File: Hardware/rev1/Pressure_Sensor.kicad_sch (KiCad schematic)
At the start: 4 parts, among them U3 MS5607-02BA

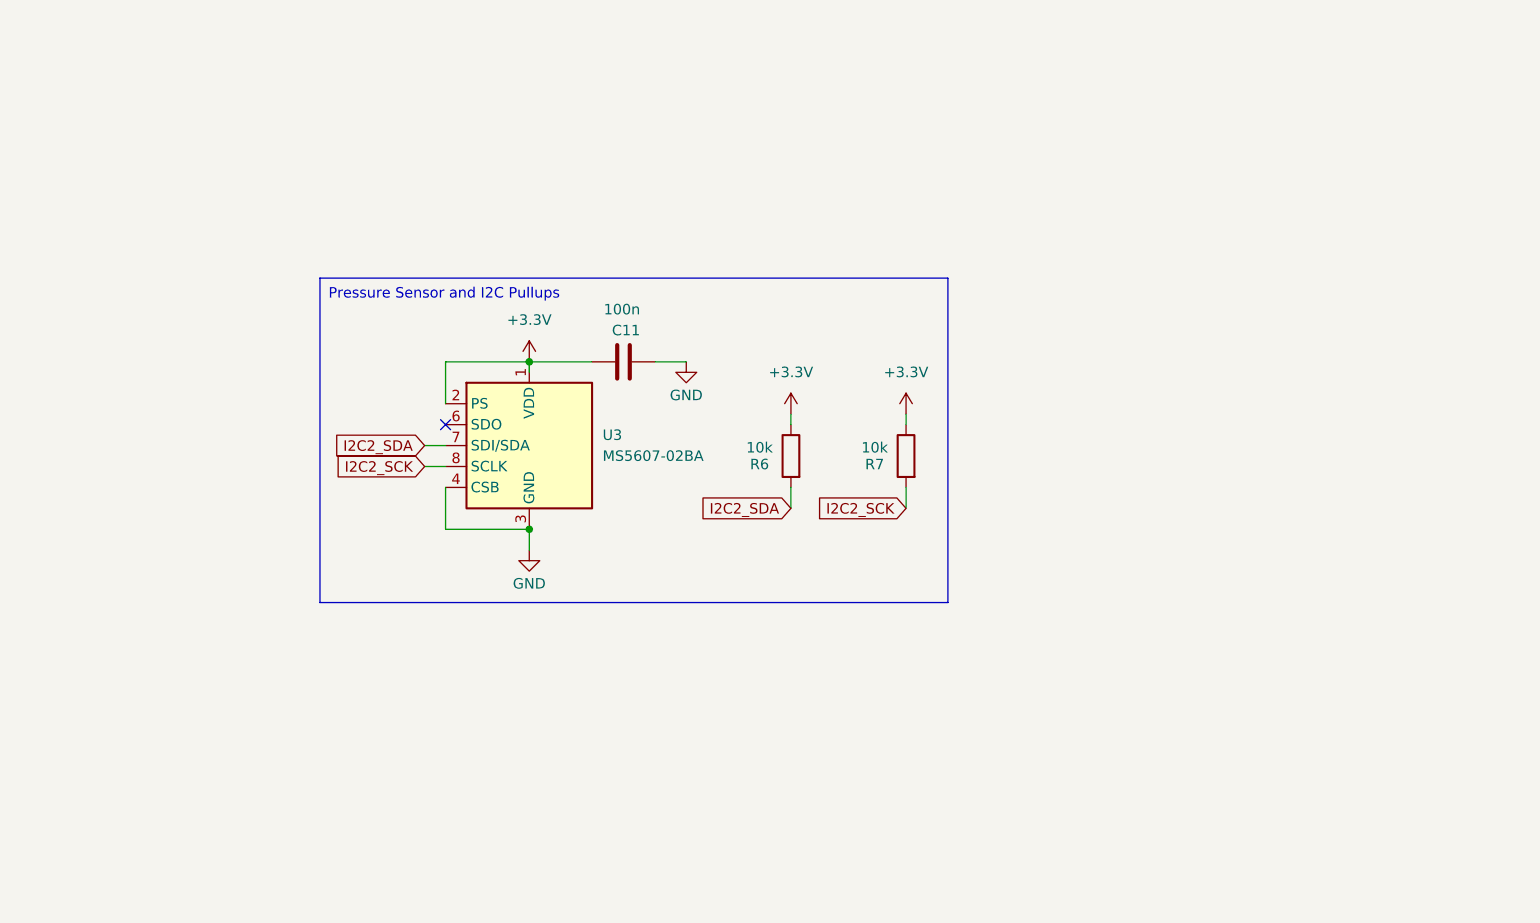
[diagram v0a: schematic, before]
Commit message: Add buses (maybe)
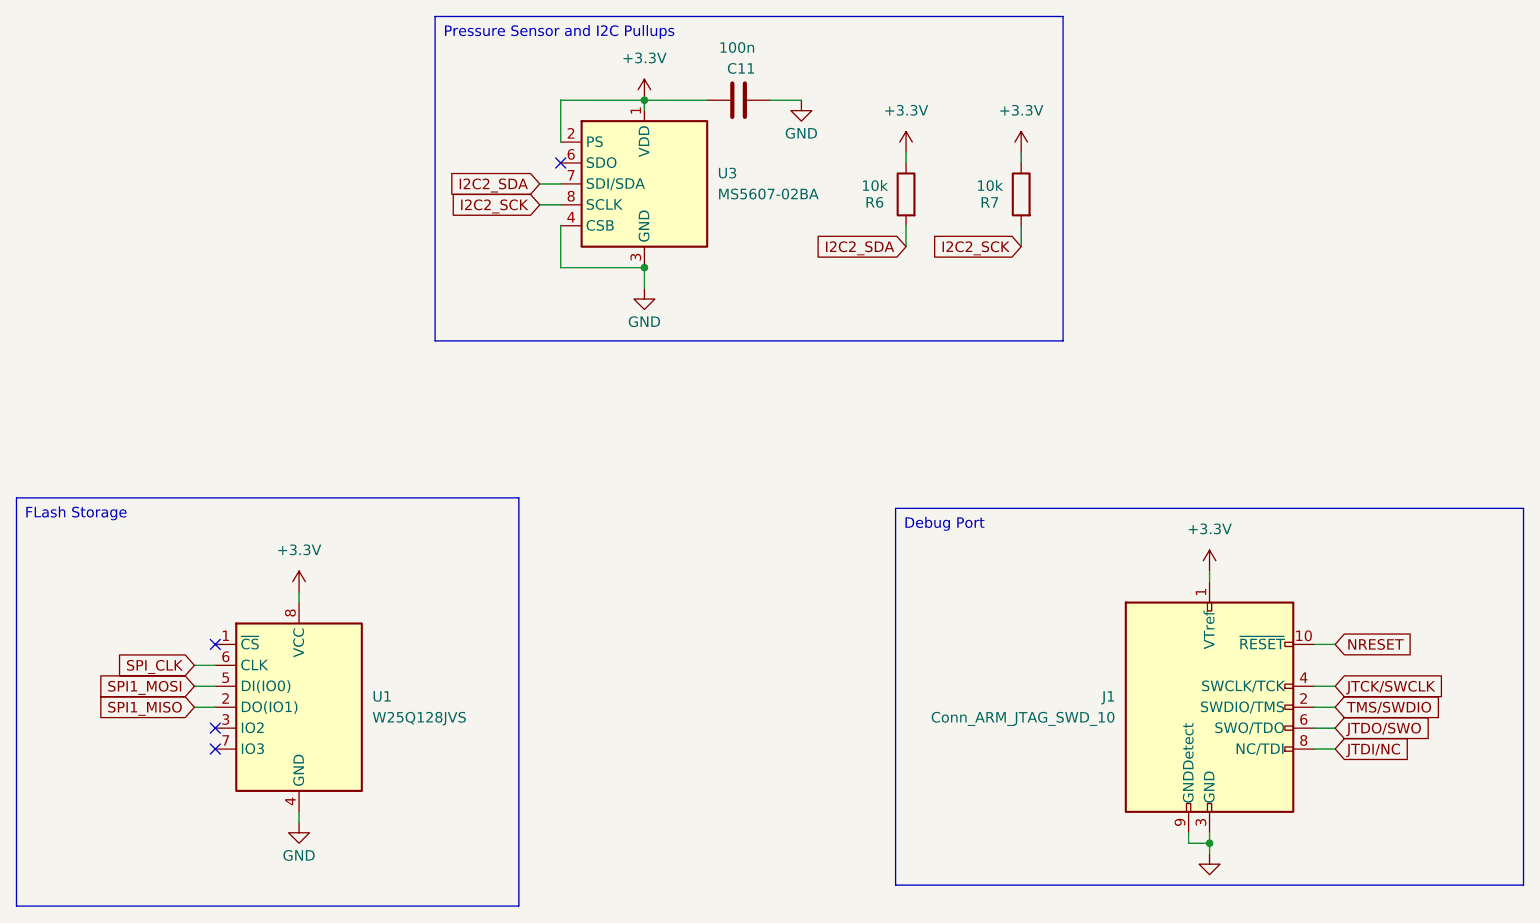
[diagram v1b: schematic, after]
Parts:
- added J1: Conn_ARM_JTAG_SWD_10, symbol Connector:Conn_ARM_JTAG_SWD_10
- added U1: W25Q128JVS, Package_SO:SOIC-8_5.23x5.23mm_P1.27mm, symbol Memory_Flash:W25Q128JVS
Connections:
- net +3.3V: now also J1.1 (VTref), U1.8 (VCC)
- net GND: now also J1.3 (GND), J1.5 (GND), J1.9 (GNDDetect), U1.4 (GND)
- new net JTCK/SWCLK: J1.4 (SWCLK/TCK)
- new net JTDI/NC: J1.8 (NC/TDI)
- new net JTDO/SWO: J1.6 (SWO/TDO)
- new net NRESET: J1.10 (~{RESET})
- new net SPI1_MISO: U1.2 (DO(IO1))
- new net SPI1_MOSI: U1.5 (DI(IO0))
- new net SPI_CLK: U1.6 (CLK)
- new net TMS/SWDIO: J1.2 (SWDIO/TMS)
- no-connect marks 1 -> 4
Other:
- moved on the sheet: C11, R6, R7, U3
